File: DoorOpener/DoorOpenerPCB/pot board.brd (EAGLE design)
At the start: 26 x 34 mm, 0 parts

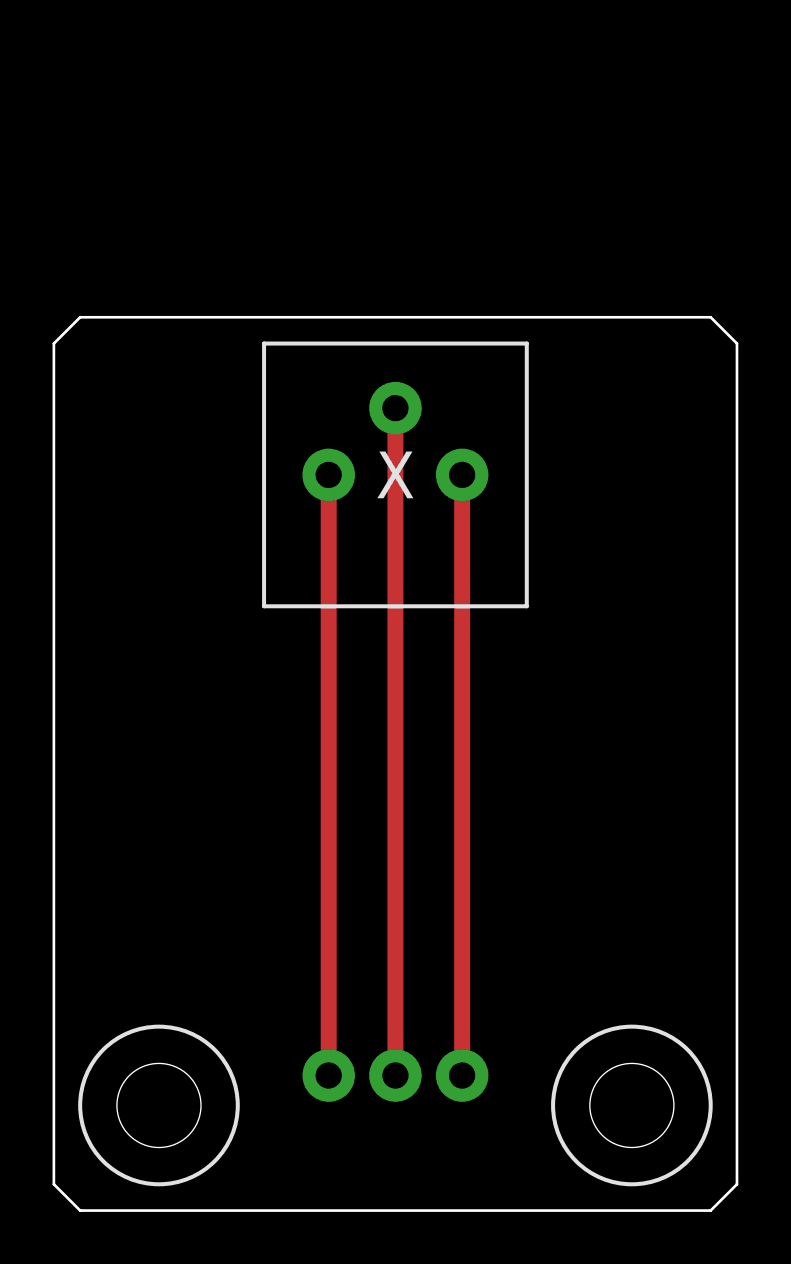
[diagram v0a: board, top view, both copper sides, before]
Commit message: board update
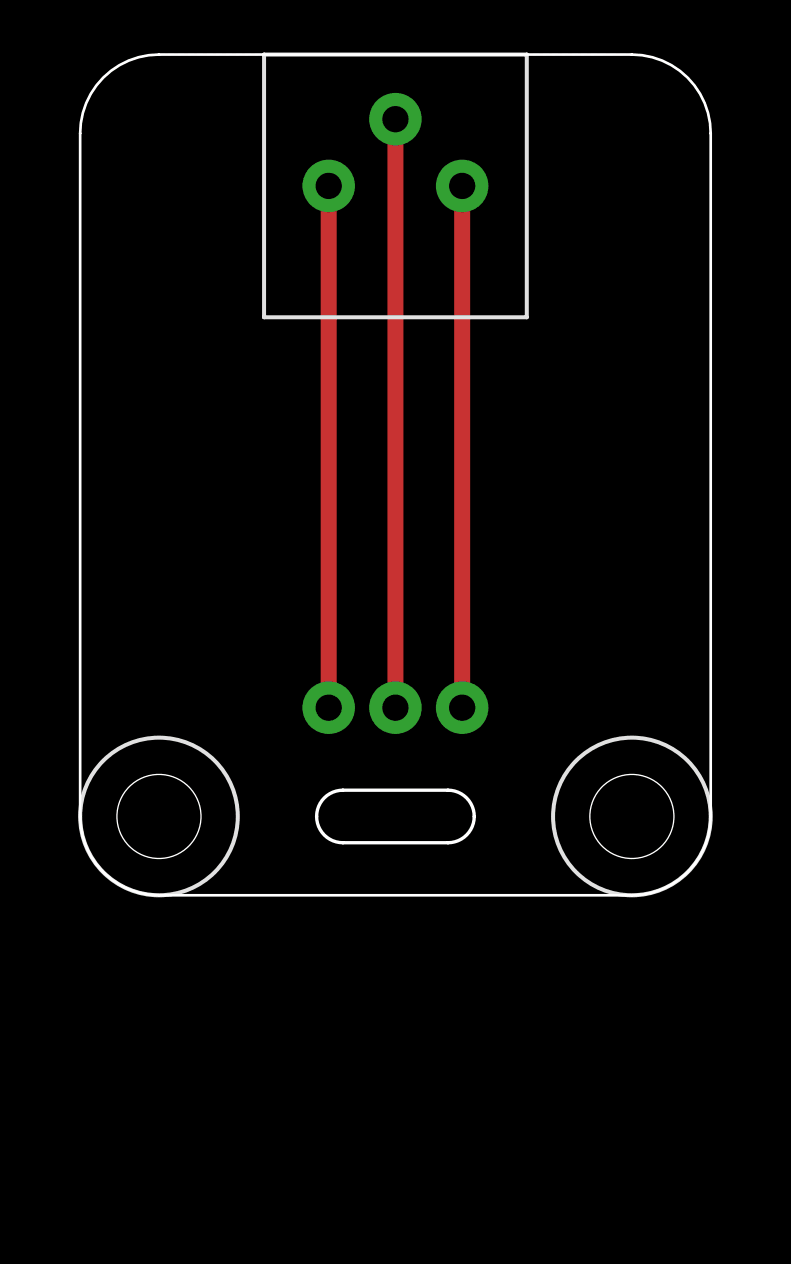
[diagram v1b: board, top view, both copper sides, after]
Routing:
- net 3: track 22.9 -> 19.9 mm
- net 2: track 25.4 -> 22.4 mm
- net 1: track 22.9 -> 19.9 mm
- added copper zone on layer 16, net S$2
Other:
- board size 26 x 34 mm -> 24 x 32 mm
- board text removed: "Luca Anastasio FabLabAQ"
- board text removed: "X"
